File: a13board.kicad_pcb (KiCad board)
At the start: 4 copper layers, 122.3 x 91.1 mm, 152 parts, among them P1 CONN_20, P2 CONN_20, P3 CONN_20, P4 CONN_20, P5 CONN_20, U1 H27UBG8T2A/TSOP48, U2 A13, U3 H5TQ2G43CFR, U4 H5TQ2G43CFR, U5 OLIMEX_IC_AXP209, U6 SY8008BAAC, U7 SY8008BAAC

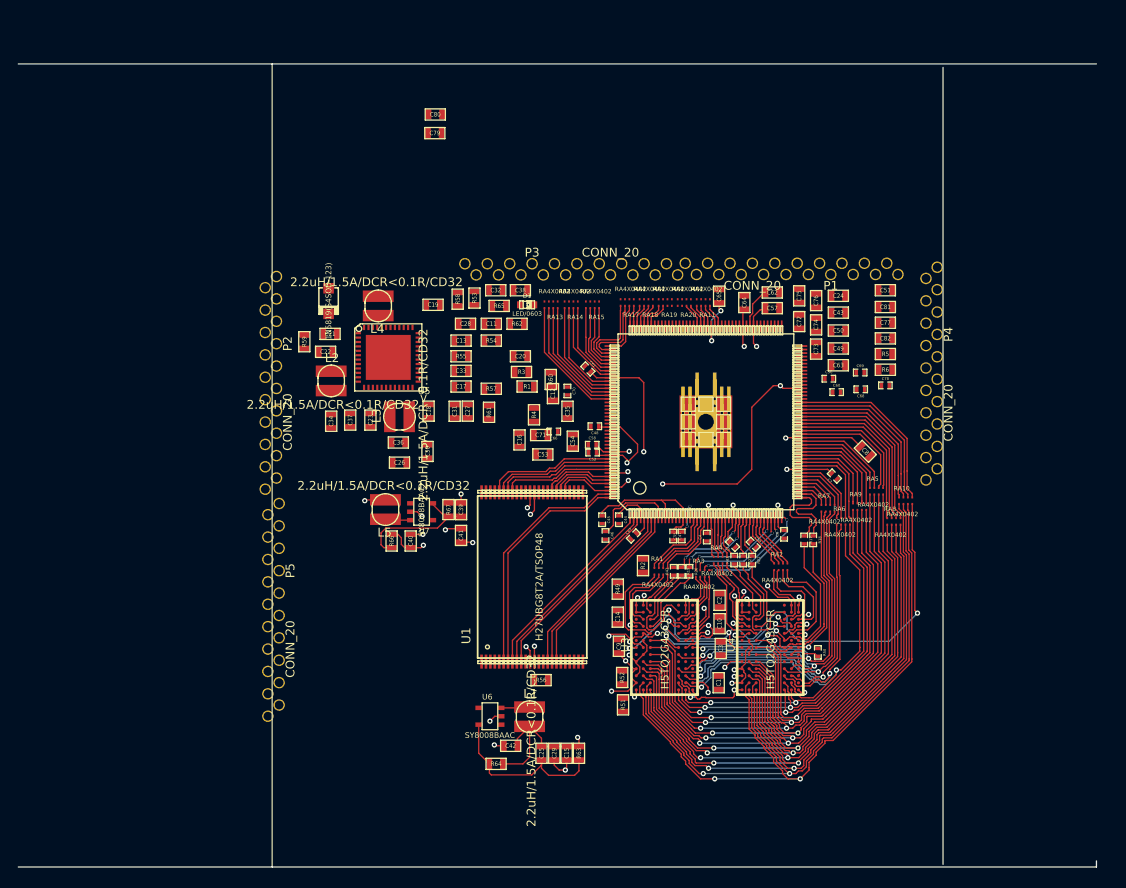
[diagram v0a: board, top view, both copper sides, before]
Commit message: Meeting 5x10 goal
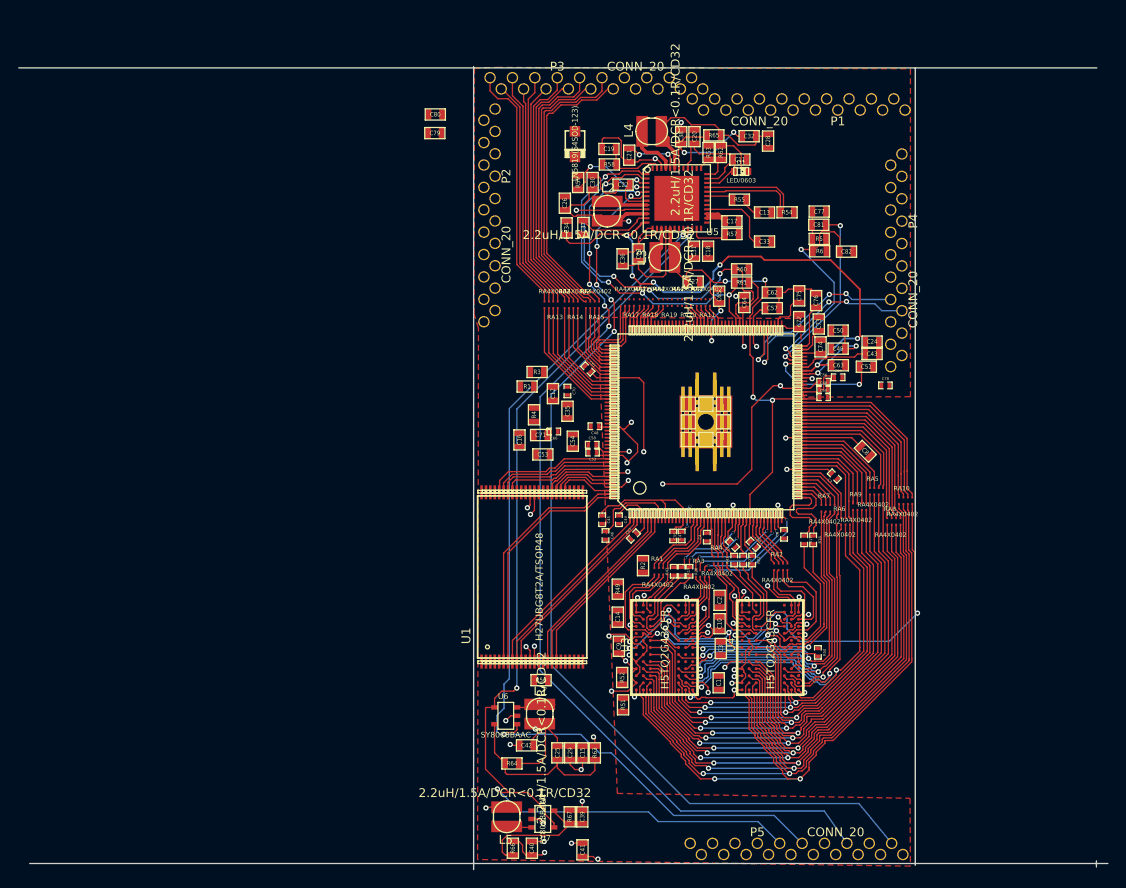
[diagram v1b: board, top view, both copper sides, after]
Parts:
- moved P5 65.9 mm to (125.0, 139.4), turned to 180 degrees
- moved C28 40.1 mm to (120.5, 59.1), turned to 90 degrees
- moved C21 39.5 mm to (104.8, 60.8), turned to 270 degrees
- moved C22 38.7 mm to (104.1, 64.1)
- moved C41 38.2 mm to (99.5, 139.6)
- moved C40 37.5 mm to (93.8, 139.4)
- moved L5 37.5 mm to (90.9, 135.8)
- moved R66 37.5 mm to (91.6, 139.4)
- moved R67 37.5 mm to (98.0, 135.8)
- moved U7 37.5 mm to (95.0, 136.1)
- moved C39 37.5 mm to (99.5, 135.8)
- moved C33 37.4 mm to (120.2, 70.5)
- moved U5 37.4 mm to (110.2, 65.7)
- moved C13 37.4 mm to (120.2, 67.2)
- moved L4 36.8 mm to (107.3, 58.0), turned to 90 degrees
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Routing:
- net RESET_SW: track 0.00 -> 157.4 mm, vias 0 -> 5
- net EXTEN: track 0.00 -> 108.0 mm, vias 0 -> 2
- net USB0-DRV: track 0.00 -> 107.9 mm, vias 0 -> 5
- net PIN2: track 0.00 -> 107.5 mm, vias 0 -> 5
- net VPP: track 0.00 -> 65.0 mm, vias 0 -> 6
- net /power/VDD_INT: track 13.9 -> 66.7 mm, vias 2 -> 6
- net GND: track 67.4 -> 113.2 mm, vias 27 -> 32
- net TWI0_SCK: track 0.00 -> 45.6 mm, vias 0 -> 4
- net TWI0_SDA: track 0.00 -> 40.7 mm, vias 0 -> 4
- net PD14: track 0.00 -> 33.2 mm
- net PD15: track 0.00 -> 32.8 mm
- net PD12: track 0.00 -> 31.2 mm
- net PD13: track 0.00 -> 30.9 mm
- net PD10: track 0.00 -> 28.9 mm
- net PD2: track 0.00 -> 28.6 mm
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- added copper zone on F.Cu, net GND
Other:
- board size 122.3 x 91.1 mm -> 123.5 x 91.1 mm
- net class power: clearance 2 -> 0.2; trace_width 0.2 -> 0.4
- rule solder_mask_min_width: 0.1 -> 0.3
